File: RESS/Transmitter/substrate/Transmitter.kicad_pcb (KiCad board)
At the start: 2 copper layers, 42 x 45 mm, 14 parts, among them J3 ADP_L, J4 ADP_R, J5 POWER, J6 ESS_IN, SW1 SW_SPDT

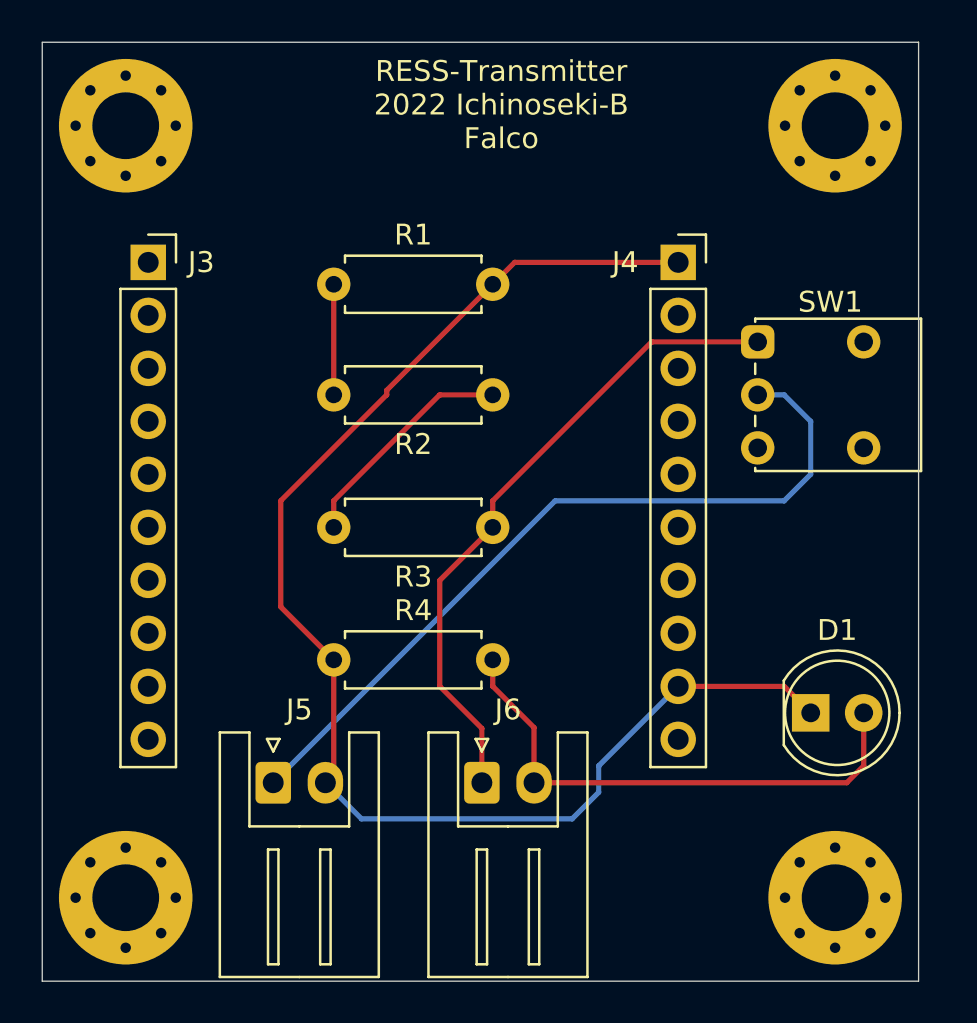
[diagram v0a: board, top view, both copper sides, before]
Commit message: 回路の細かな修正
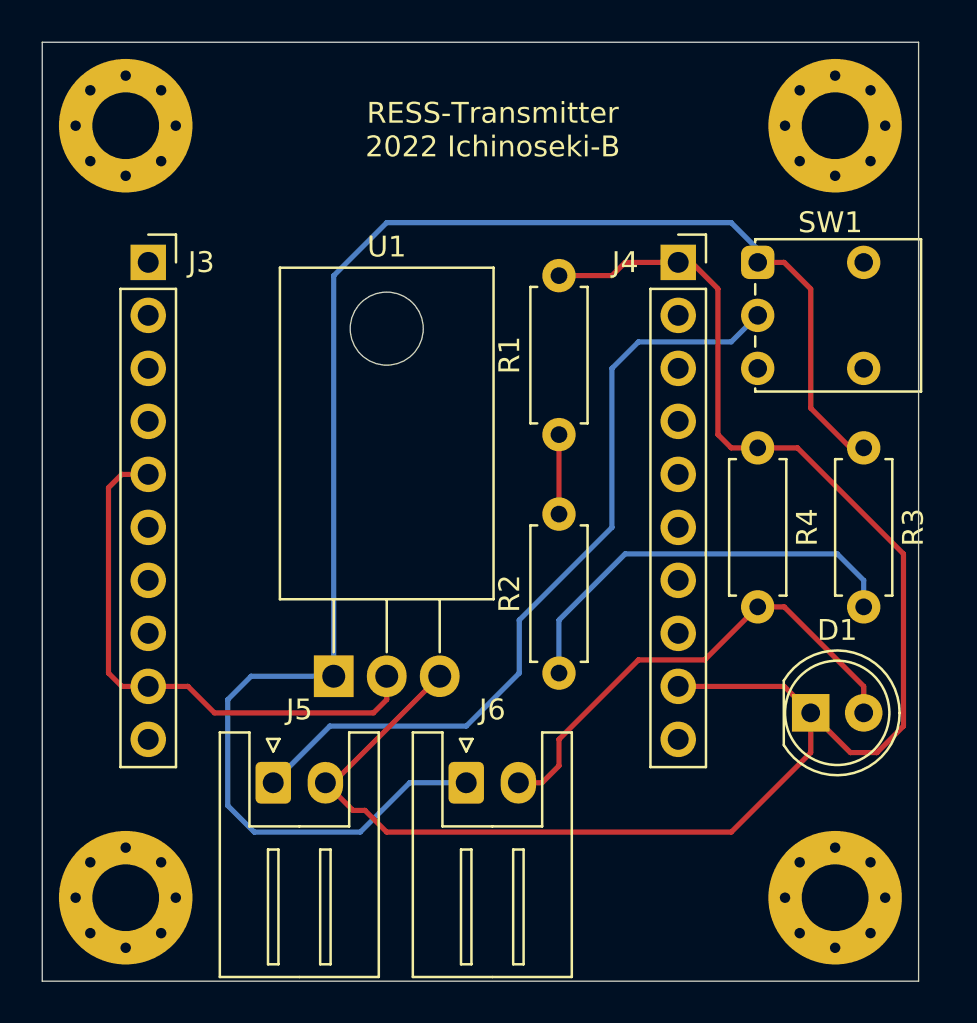
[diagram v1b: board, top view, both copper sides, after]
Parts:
- added U1: TA48033S, Package_TO_SOT_THT:TO-220-3_Horizontal_TabDown, F.Cu at (141.0, 102.4)
- moved R4 22.7 mm to (161.3, 91.4), turned to 270 degrees
- moved R3 18.2 mm to (166.4, 91.4), turned to 270 degrees
- moved R2 13.7 mm to (151.8, 102.2), turned to 90 degrees
- moved R1 13.0 mm to (151.8, 90.8), turned to 90 degrees
- moved SW1 3.81 mm to (161.3, 82.5)
- moved J6 0.75 mm to (147.3, 107.5)
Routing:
- net +5V: track 31.3 -> 77.4 mm
- net +3V3: track 0.00 -> 26.6 mm
- net ESS: track 66.5 -> 82.9 mm
- net Net-(R2-Pad1): track 11.0 -> 20.3 mm
- net LED: track 25.4 -> 23.6 mm
- net Net-(R1-Pad1): track 5.30 -> 3.81 mm
- net PW_IN: track 37.5 -> 38.4 mm
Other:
- board text added: "RESS-Transmitter 2022 Ichinoseki-B"
- board text removed: "RESS-Transmitter 2022 Ichinoseki-B Falco"
